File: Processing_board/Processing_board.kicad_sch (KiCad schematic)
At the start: 26 parts, among them J1 Conn_01x08_Pin, J2 Conn_01x08_Pin, J3 Conn_01x06_Pin, J4 Conn_01x03_Pin, J5 Conn_01x03_Pin, J6 Conn_01x02_Pin, J7 Conn_01x02_Pin, SW1 TL3305BF100QG, SW2 TL3305BF100QG, U1 STM32WBA63CIU6

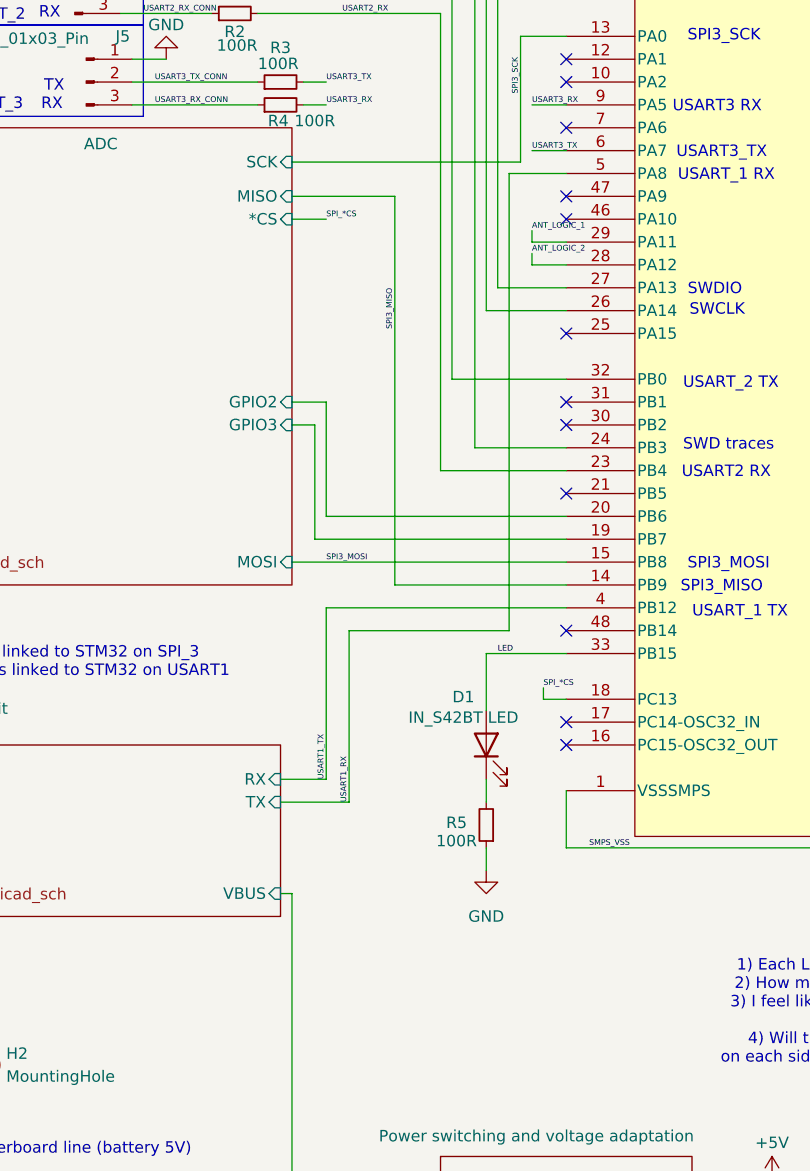
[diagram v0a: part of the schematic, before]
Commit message: more progress
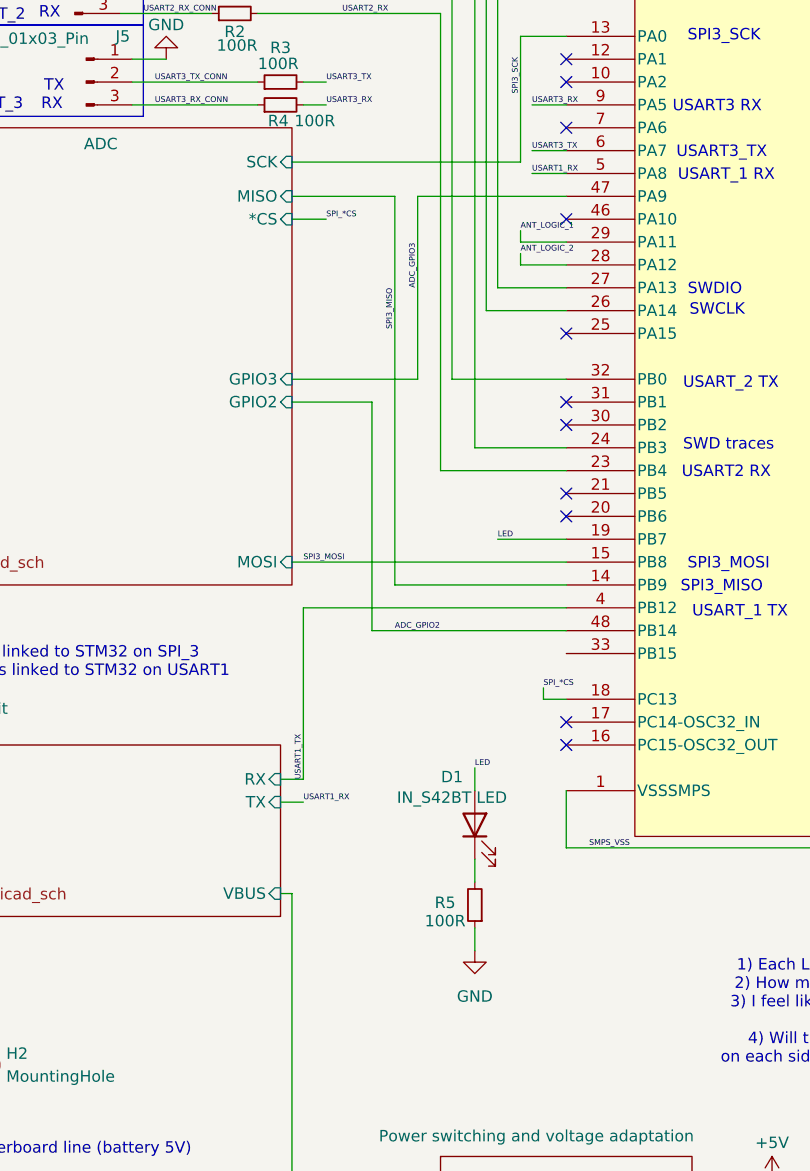
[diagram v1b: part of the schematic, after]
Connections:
- net ADC/GPIO3 is gone; now on net LED: U1.19 (PB7)
- net LED: no longer U1.33 (PB15)
- net ADC_GPIO3: now reaches U1.47 (PA9)
- net ADC_GPIO2: now reaches U1.48 (PB14)
- net ADC/GPIO2: no longer names the net of U1.20 (PB6)
- no-connect marks 16 -> 15
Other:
- moved on the sheet: D1, R5
